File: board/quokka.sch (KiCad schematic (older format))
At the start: 0 parts

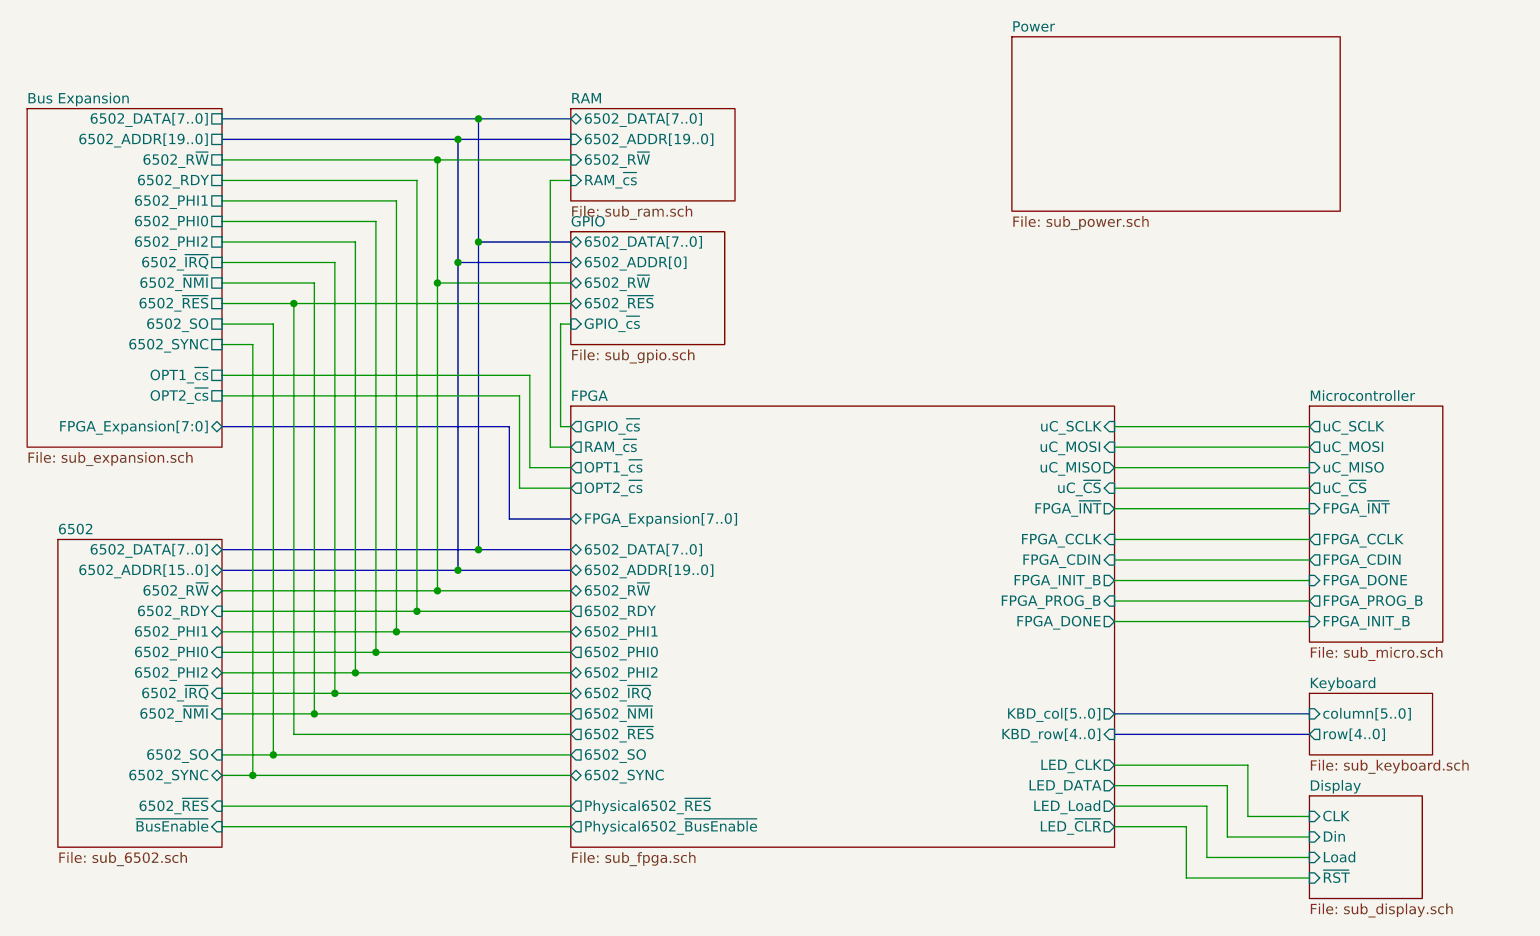
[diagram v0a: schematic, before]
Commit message: gpio done
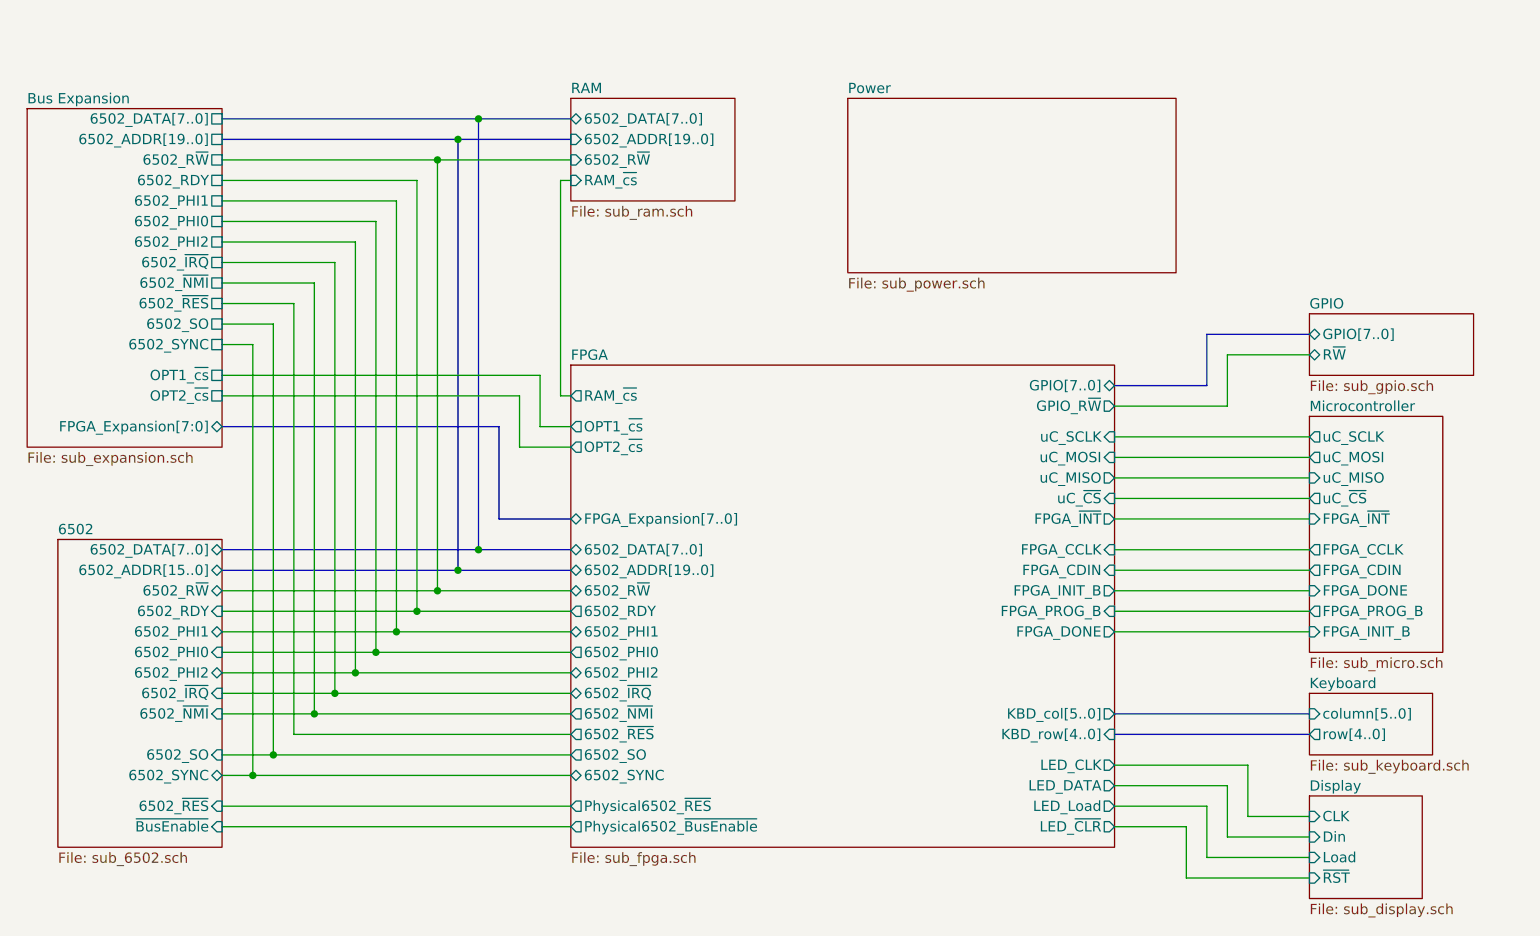
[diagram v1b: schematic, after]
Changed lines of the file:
@@
 $EndDescr
 $Sheet
-S 6900 1450 1600 850
+S 6100 1750 1600 850
 U 5A9C14CE
 F0 "Power" 50
@@
 $EndSheet
 $Sheet
-S 8350 3250 650  1150
+S 8350 3300 650  1150
 U 5A9C14E5
 F0 "Microcontroller" 50
 F1 "sub_micro.sch" 50
-F2 "uC_SCLK" O L 8350 3350 50
-F3 "uC_MOSI" O L 8350 3450 50
-F4 "uC_MISO" I L 8350 3550 50
-F5 "uC_~CS" O L 8350 3650 50
-F6 "FPGA_~INT" I L 8350 3750 50
-F7 "FPGA_CCLK" O L 8350 3900 50
-F8 "FPGA_CDIN" O L 8350 4000 50
-F9 "FPGA_DONE" I L 8350 4100 50
-F10 "FPGA_PROG_B" O L 8350 4200 50
-F11 "FPGA_INIT_B" I L 8350 4300 50
-$EndSheet
-$Sheet
-S 4750 2400 750  550
+F2 "uC_SCLK" O L 8350 3400 50
+F3 "uC_MOSI" O L 8350 3500 50
+F4 "uC_MISO" I L 8350 3600 50
+F5 "uC_~CS" O L 8350 3700 50
+F6 "FPGA_~INT" I L 8350 3800 50
+F7 "FPGA_CCLK" O L 8350 3950 50
+F8 "FPGA_CDIN" O L 8350 4050 50
+F9 "FPGA_DONE" I L 8350 4150 50
+F10 "FPGA_PROG_B" O L 8350 4250 50
+F11 "FPGA_INIT_B" I L 8350 4350 50
+$EndSheet
+$Sheet
+S 8350 2800 800  300
 U 5A9C14FD
 F0 "GPIO" 50
 F1 "sub_gpio.sch" 50
-F2 "6502_DATA[7..0]" T L 4750 2450 50
-F3 "6502_R~W" B L 4750 2650 50
-F4 "6502_ADDR[0]" B L 4750 2550 50
-F5 "GPIO_~cs" I L 4750 2850 50
-F6 "6502_~RES" B L 4750 2750 50
+F2 "R~W" B L 8350 3000 50
+F3 "GPIO[7..0]" B L 8350 2900 50
 $EndSheet
 $Sheet
@@
 $EndSheet
 $Sheet
-S 4750 1800 800  450
+S 4750 1750 800  500
 U 5AA3897D
 F0 "RAM" 50
@@
 Wire Bus Line
 	4300 3950 3050 3950
-Wire Bus Line
-	4750 1850 4300 1850
-Wire Bus Line
-	4750 2450 4300 2450
-Wire Bus Line
-	4750 2550 4200 2550
-Wire Bus Line
-	4750 1950 4200 1950
-Wire Wire Line
-	4750 2050 4100 2050
-Wire Wire Line
-	4750 2650 4100 2650
-Connection ~ 4100 2050
-Connection ~ 4100 2650
-Connection ~ 4200 1950
-Connection ~ 4200 2550
-Connection ~ 4300 1850
-Connection ~ 4300 2450
-Wire Wire Line
-	4100 2650 4100 4150
-Wire Bus Line
-	4200 2550 4200 4050
-Wire Bus Line
-	4300 1850 4300 2450
-Wire Bus Line
-	4300 2450 4300 3950
-Wire Bus Line
-	4200 1950 4200 2550
-Wire Wire Line
-	4100 2050 4100 2650
 Wire Wire Line
 	3050 5200 4750 5200
@@
 	3050 5300 4750 5300
 Wire Wire Line
-	4750 2750 3400 2750
-Connection ~ 3400 2750
-Wire Wire Line
-	4750 3350 4700 3350
-Wire Wire Line
-	4700 3350 4700 2850
-Wire Wire Line
-	4700 2850 4750 2850
-Wire Wire Line
-	4750 3450 4650 3450
-Wire Wire Line
-	4650 3450 4650 2150
-Wire Wire Line
-	4650 2150 4750 2150
-Wire Wire Line
-	4750 3550 4550 3550
-Wire Wire Line
-	4550 3550 4550 3100
-Wire Wire Line
-	4550 3100 3050 3100
+	4750 3350 4600 3350
+Wire Wire Line
+	4600 3350 4600 3100
+Wire Wire Line
+	4600 3100 3050 3100
 Wire Wire Line
 	3050 3200 4500 3200
 Wire Wire Line
-	4500 3200 4500 3650
-Wire Wire Line
-	4500 3650 4750 3650
-Wire Bus Line
-	4750 3800 4450 3800
-Wire Bus Line
-	4450 3800 4450 3350
-Wire Bus Line
-	3050 3350 4450 3350
-$Sheet
-S 4750 3250 2650 2150
+	4500 3200 4500 3450
+Wire Wire Line
+	4500 3450 4750 3450
+Wire Bus Line
+	4750 3800 4400 3800
+Wire Bus Line
+	4400 3800 4400 3350
+Wire Bus Line
+	3050 3350 4400 3350
+$Sheet
+S 4750 3050 2650 2350
 U 5A9C14F1
 F0 "FPGA" 50
@@
 F4 "6502_DATA[7..0]" T L 4750 3950 50
 F5 "6502_ADDR[19..0]" B L 4750 4050 50
-F6 "RAM_~cs" O L 4750 3450 50
-F7 "GPIO_~cs" O L 4750 3350 50
-F8 "OPT1_~cs" O L 4750 3550 50
-F9 "OPT2_~cs" O L 4750 3650 50
-F10 "FPGA_Expansion[7..0]" B L 4750 3800 50
-F11 "LED_CLK" O R 7400 5000 50
-F12 "LED_DATA" O R 7400 5100 50
-F13 "LED_Load" O R 7400 5200 50
-F14 "6502_R~W" B L 4750 4150 50
-F15 "6502_RDY" O L 4750 4250 50
-F16 "6502_PHI1" B L 4750 4350 50
-F17 "6502_PHI0" O L 4750 4450 50
-F18 "6502_PHI2" B L 4750 4550 50
-F19 "6502_~IRQ" B L 4750 4650 50
-F20 "6502_~NMI" O L 4750 4750 50
-F21 "Physical6502_~RES" O L 4750 5200 50
-F22 "6502_SO" O L 4750 4950 50
-F23 "6502_SYNC" B L 4750 5050 50
-F24 "6502_~RES" O L 4750 4850 50
-F25 "Physical6502_~BusEnable" O L 4750 5300 50
-F26 "uC_SCLK" I R 7400 3350 50
-F27 "uC_MOSI" I R 7400 3450 50
-F28 "uC_MISO" O R 7400 3550 50
-F29 "uC_~CS" I R 7400 3650 50
-F30 "FPGA_~INT" O R 7400 3750 50
-F31 "FPGA_CCLK" I R 7400 3900 50
-F32 "FPGA_CDIN" I R 7400 4000 50
-F33 "LED_~CLR" O R 7400 5300 50
-F34 "FPGA_INIT_B" O R 7400 4100 50
-F35 "FPGA_DONE" O R 7400 4300 50
-F36 "FPGA_PROG_B" I R 7400 4200 50
-$EndSheet
-Wire Wire Line
-	8350 3350 7400 3350
-Wire Wire Line
-	7400 3450 8350 3450
-Wire Wire Line
-	8350 3550 7400 3550
-Wire Wire Line
-	7400 3650 8350 3650
-Wire Wire Line
-	8350 3750 7400 3750
-Wire Wire Line
-	7400 3900 8350 3900
-Wire Wire Line
-	8350 4000 7400 4000
+F6 "RAM_~cs" O L 4750 3200 50
+F7 "OPT1_~cs" O L 4750 3350 50
+F8 "OPT2_~cs" O L 4750 3450 50
+F9 "FPGA_Expansion[7..0]" B L 4750 3800 50
+F10 "LED_CLK" O R 7400 5000 50
+F11 "LED_DATA" O R 7400 5100 50
+F12 "LED_Load" O R 7400 5200 50
+F13 "6502_R~W" B L 4750 4150 50
+F14 "6502_RDY" O L 4750 4250 50
+F15 "6502_PHI1" B L 4750 4350 50
+F16 "6502_PHI0" O L 4750 4450 50
+F17 "6502_PHI2" B L 4750 4550 50
+F18 "6502_~IRQ" B L 4750 4650 50
+F19 "6502_~NMI" O L 4750 4750 50
+F20 "Physical6502_~RES" O L 4750 5200 50
+F21 "6502_SO" O L 4750 4950 50
+F22 "6502_SYNC" B L 4750 5050 50
+F23 "6502_~RES" O L 4750 4850 50
+F24 "Physical6502_~BusEnable" O L 4750 5300 50
+F25 "uC_SCLK" I R 7400 3400 50
+F26 "uC_MOSI" I R 7400 3500 50
+F27 "uC_MISO" O R 7400 3600 50
+F28 "uC_~CS" I R 7400 3700 50
+F29 "FPGA_~INT" O R 7400 3800 50
+F30 "FPGA_CCLK" I R 7400 3950 50
+F31 "FPGA_CDIN" I R 7400 4050 50
+F32 "LED_~CLR" O R 7400 5300 50
+F33 "FPGA_INIT_B" O R 7400 4150 50
+F34 "FPGA_DONE" O R 7400 4350 50
+F35 "FPGA_PROG_B" I R 7400 4250 50
+F36 "GPIO[7..0]" B R 7400 3150 50
+F37 "GPIO_R~W" O R 7400 3250 50
+$EndSheet
+Wire Wire Line
+	8350 3400 7400 3400
+Wire Wire Line
+	7400 3500 8350 3500
+Wire Wire Line
+	8350 3600 7400 3600
+Wire Wire Line
+	7400 3700 8350 3700
+Wire Wire Line
+	8350 3800 7400 3800
+Wire Wire Line
+	7400 3950 8350 3950
+Wire Wire Line
+	8350 4050 7400 4050
 Wire Bus Line
 	7400 4750 8350 4750
@@
 	7750 5550 8350 5550
 Wire Wire Line
-	8350 4100 7400 4100
-Wire Wire Line
-	7400 4200 8350 4200
-Wire Wire Line
-	8350 4300 7400 4300
+	8350 4150 7400 4150
+Wire Wire Line
+	7400 4250 8350 4250
+Wire Wire Line
+	8350 4350 7400 4350
+Wire Bus Line
+	4300 1850 4300 3950
+Wire Bus Line
+	4200 1950 4200 4050
+Wire Wire Line
+	4100 2050 4100 4150
+Wire Wire Line
+	4750 3200 4700 3200
+Wire Bus Line
+	7400 3150 7850 3150
+Wire Bus Line
+	7850 3150 7850 2900
+Wire Bus Line
+	7850 2900 8350 2900
+Wire Wire Line
+	8350 3000 7950 3000
+Wire Wire Line
+	7950 3000 7950 3250
+Wire Wire Line
+	7950 3250 7400 3250
+Wire Wire Line
+	4700 3200 4700 2150
+Wire Wire Line
+	4700 2150 4750 2150
+Connection ~ 4100 2050
+Wire Wire Line
+	4750 2050 4100 2050
+Connection ~ 4200 1950
+Wire Bus Line
+	4750 1950 4200 1950
+Connection ~ 4300 1850
+Wire Bus Line
+	4750 1850 4300 1850
 $EndSCHEMATC
